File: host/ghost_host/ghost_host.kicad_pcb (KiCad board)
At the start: 2 copper layers, 127.5 x 68.5 mm, 115 parts, among them J1 RGB_3_Pin_Connector, J10 Conn_01x06, J11 Conn_01x04, J12 RJ12_Shielded, J13 Conn_01x06, J14 Conn_01x04, J15 RJ12_Shielded, J16 Conn_01x06, J17 Conn_01x04, J18 RJ12_Shielded, J19 Conn_01x06, J2 Conn_01x04, J20 Conn_01x04, J21 RJ12_Shielded, J22 Conn_01x06, J23 RJ12_Shielded, J24 Conn_01x06, J25 Conn_01x06, J3 Conn_01x04, J4 RJ12_Shielded, J5 Conn_01x04, J6 RJ12_Shielded, J7 Conn_01x06, J8 Conn_01x04, J9 RJ12_Shielded, U1 PCA9615DP, U2 PCA9615DP, U3 PCA9615DP, U4 PCA9615DP, U5 PCA9615DP, U6 PCA9615DP, U7 PCA9615DP, U8 PCA9615DP, U9 kb2040

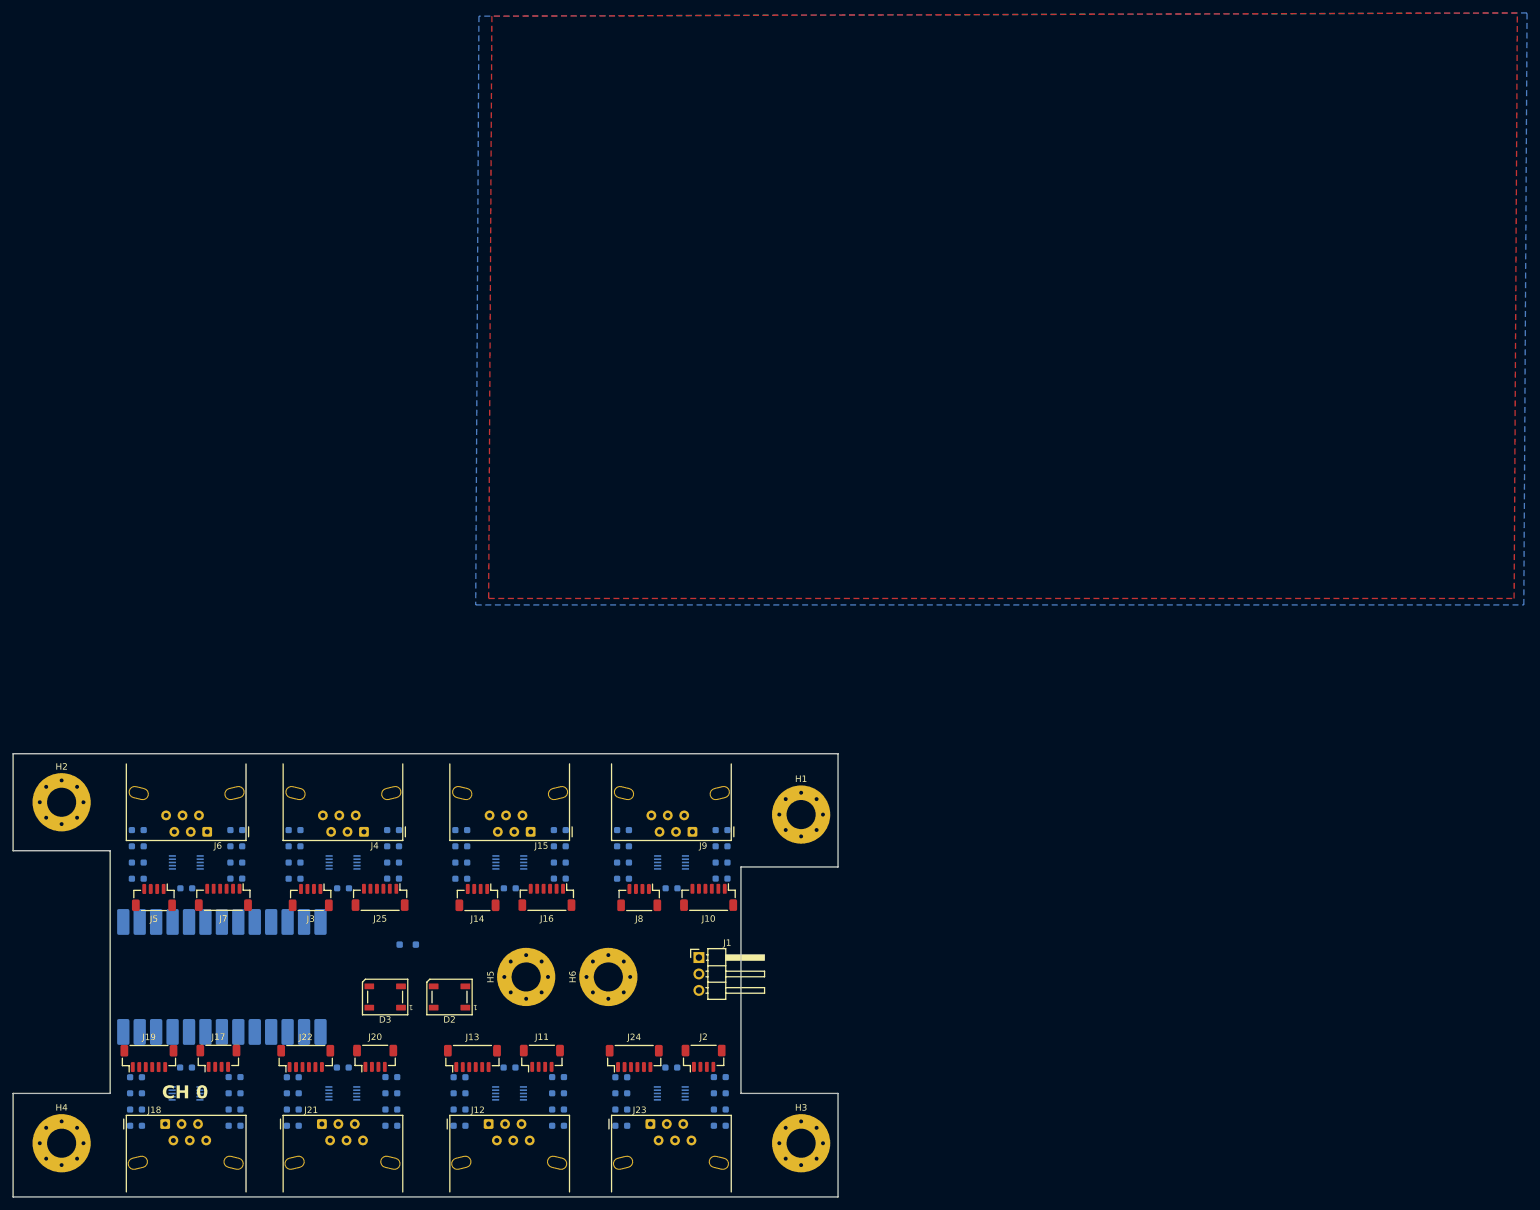
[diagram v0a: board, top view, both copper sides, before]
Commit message: finished host board
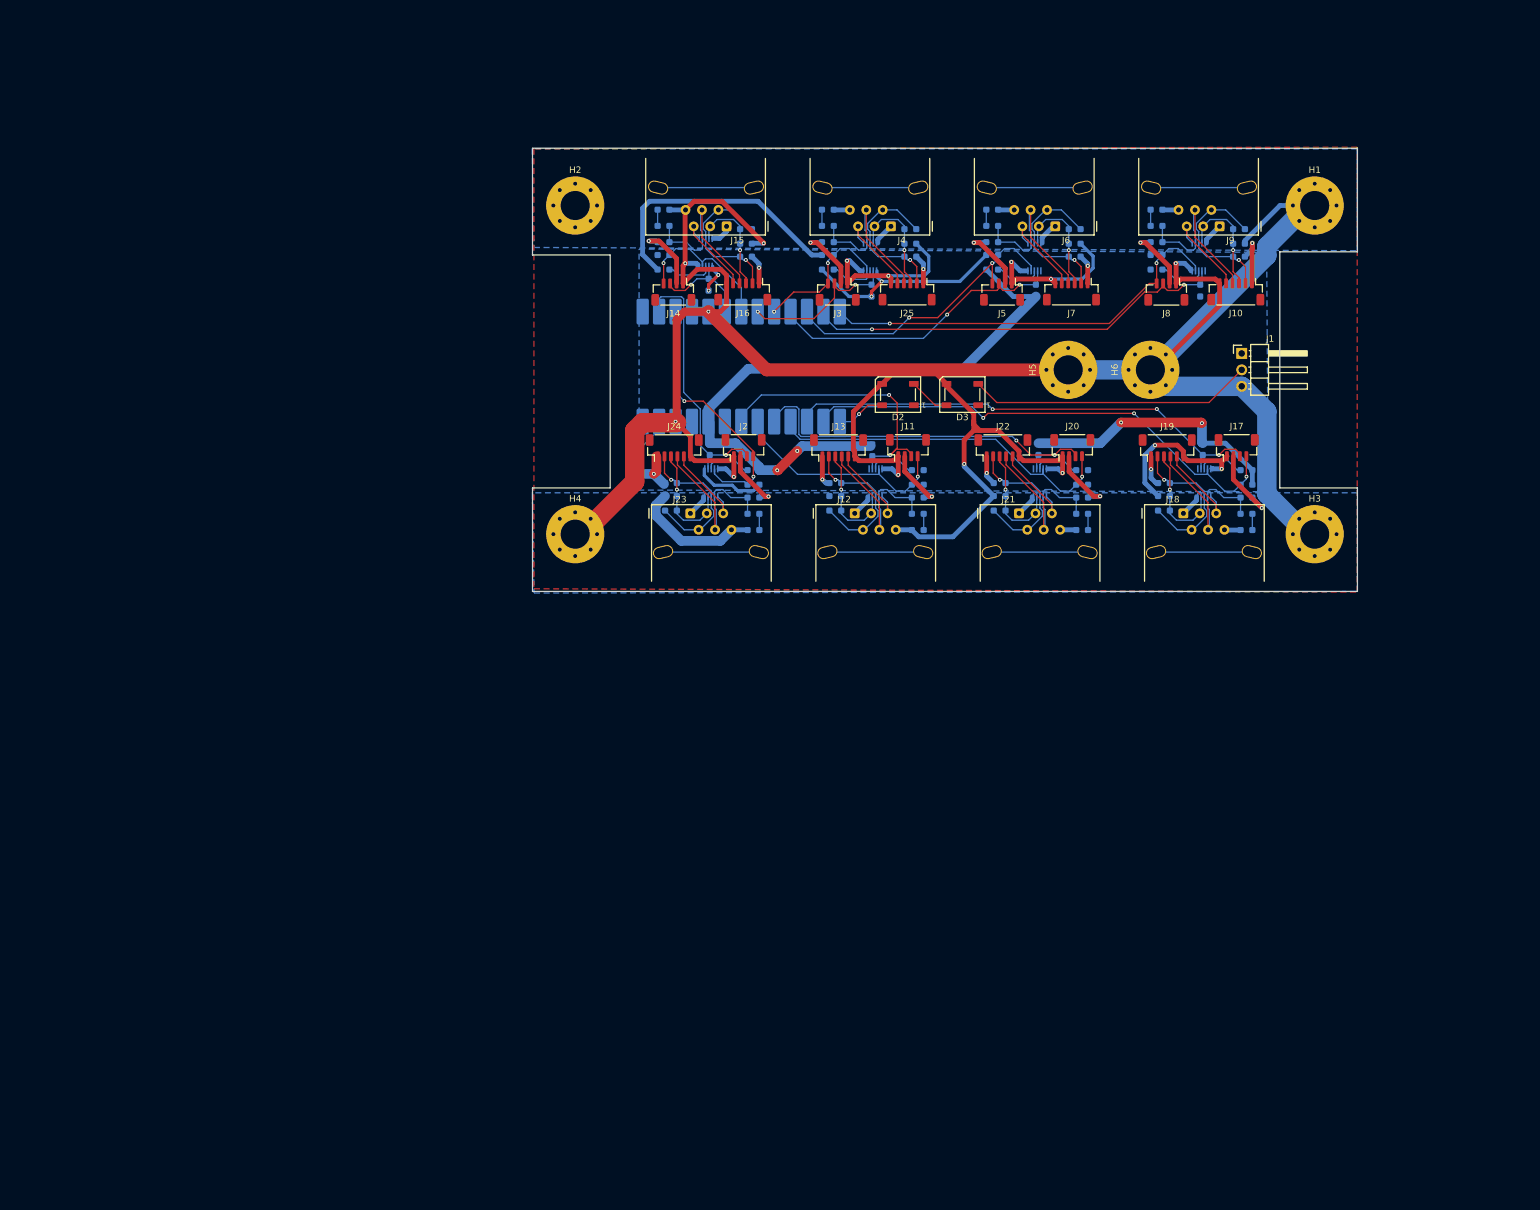
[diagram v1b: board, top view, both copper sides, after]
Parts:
- U9: value kb2040 -> ProMicro
- moved R49 199.3 mm to (190.6, 103.7), turned to 0 degrees
- moved R48 196.9 mm to (190.6, 105.9)
- moved R47 192.6 mm to (183.9, 100.4), turned to -90 degrees
- moved R50 184.1 mm to (190.6, 107.9), turned to 180 degrees
- moved J19 183.5 mm to (178.4, 100.2)
- moved J18 183.5 mm to (180.9, 110.3)
- moved U7 183.5 mm to (184.1, 105.6), turned to -90 degrees
- moved J17 183.5 mm to (189.1, 100.2)
- moved R53 183.5 mm to (177.9, 105.7)
- moved R51 181.5 mm to (190.6, 110.4)
- moved R52 179.0 mm to (190.6, 112.9), turned to 180 degrees
- moved R24 174.9 mm to (164.1, 68.7), turned to 0 degrees
- moved R54 173.9 mm to (177.9, 109.9)
- moved R23 171.0 mm to (164.1, 66.4)
- moved R55 169.4 mm to (177.9, 107.7), turned to 180 degrees
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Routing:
- net GND: track 0.00 -> 537.0 mm, vias 0 -> 15
- net +3.3V: track 0.00 -> 232.3 mm, vias 0 -> 8
- net +5V: track 0.00 -> 157.1 mm, vias 0 -> 16
- net /scl8: track 0.00 -> 78.6 mm, vias 0 -> 3
- net /sda8: track 0.00 -> 75.7 mm, vias 0 -> 3
- net /sda5: track 0.00 -> 66.3 mm, vias 0 -> 2
- net /scl5: track 0.00 -> 64.5 mm, vias 0 -> 2
- net /sda7: track 0.00 -> 59.6 mm, vias 0 -> 2
- net /scl7: track 0.00 -> 56.2 mm, vias 0 -> 1
- net /sda4: track 0.00 -> 49.0 mm, vias 0 -> 2
- net /scl4: track 0.00 -> 48.7 mm, vias 0 -> 2
- net /sda6: track 0.00 -> 44.5 mm, vias 0 -> 2
- net Net-(D3-DOUT): track 0.00 -> 44.0 mm
- net /scl1: track 0.00 -> 41.2 mm, vias 0 -> 2
- net /sda1: track 0.00 -> 40.9 mm, vias 0 -> 1
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- added copper zone on F.Cu, net +5V
- added copper zone on B.Cu, net GND
- removed copper zone on F.Cu, net GND
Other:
- outline, holes or cut-outs redrawn
- board text removed: "CH 0"
